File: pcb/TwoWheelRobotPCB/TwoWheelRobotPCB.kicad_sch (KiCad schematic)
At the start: 30 parts, among them J1 Motor1, J2 Motor2, J3 L298n_sense_connector, J4 ACS712_connector, U1 NodeMCU1.0(ESP-12E), U2 L298HN, U3 ACS712_M1, U4 TXB0104D, U5 ACS712_M2, U6 MCP3004

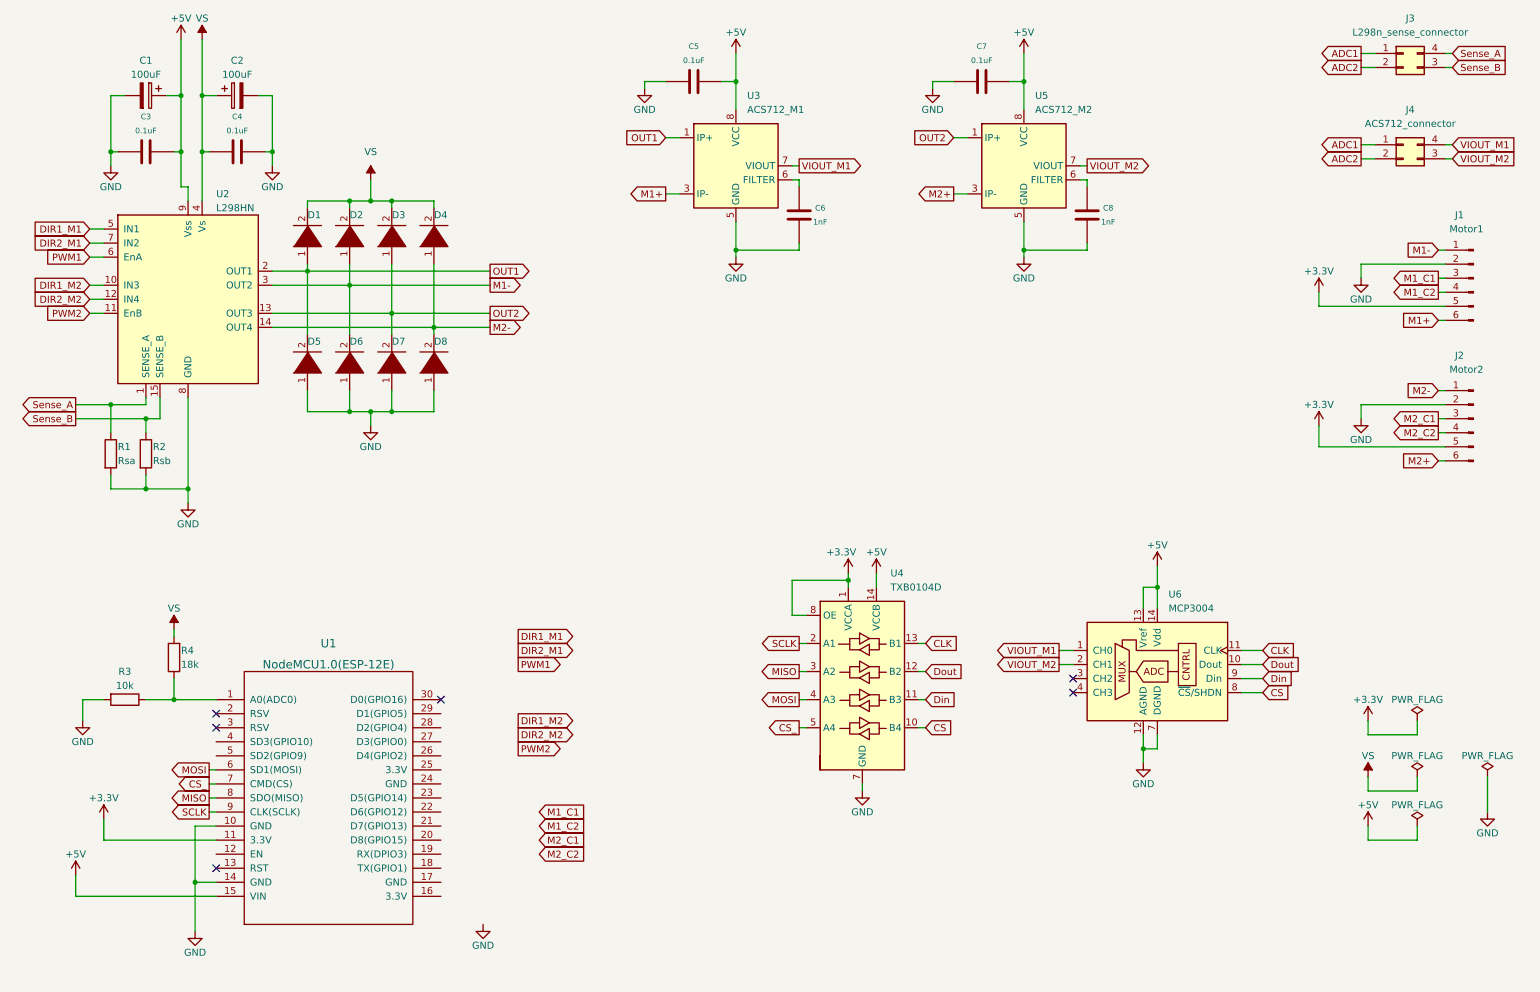
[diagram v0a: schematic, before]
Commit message: pcb update
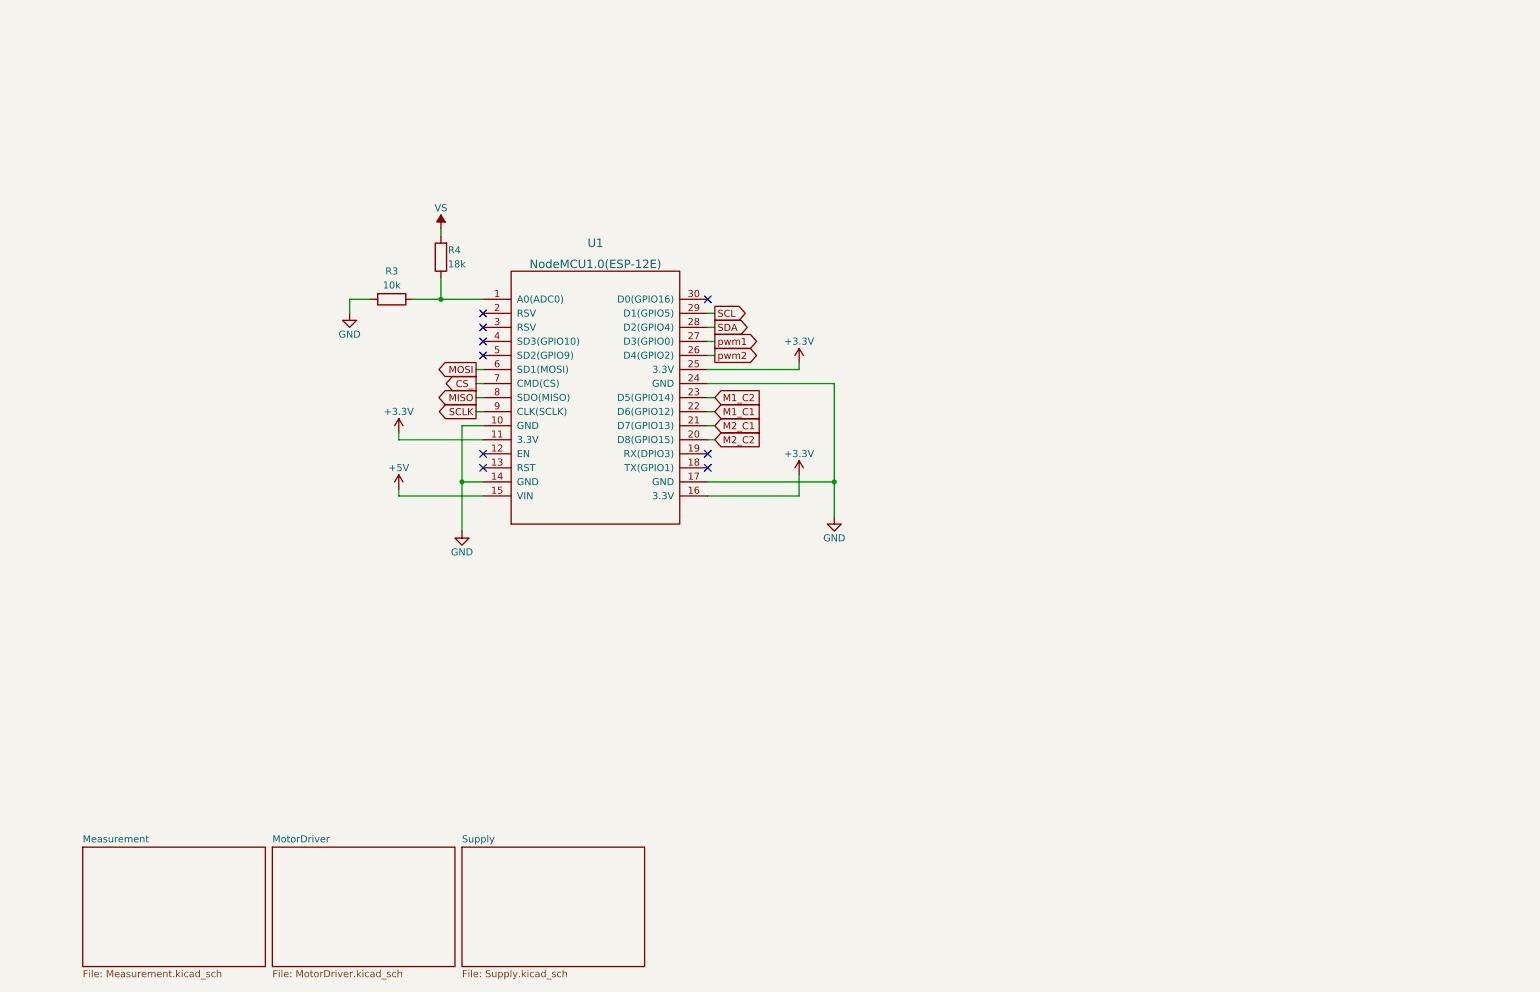
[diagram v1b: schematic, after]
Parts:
- removed C1, C2: 100uF, symbol Device:C_Polarized
- removed C3, C4, C5, C7: 0.1uF, symbol cyclophone:C
- removed C6, C8: 1nF, symbol cyclophone:C
- removed D1, D2, D3, D4, D5, D6, D7, D8: DIODE, symbol pspice:DIODE
- removed J1: Motor1, Connector_PinHeader_2.54mm:PinHeader_1x06_P2.54mm_Vertical, symbol Connector:Conn_01x06_Male
- removed J2: Motor2, Connector_PinHeader_2.54mm:PinHeader_1x06_P2.54mm_Vertical, symbol Connector:Conn_01x06_Male
- removed J3: L298n_sense_connector, Connector_PinHeader_2.54mm:PinHeader_2x02_P2.54mm_Vertical, symbol Connector_Generic:Conn_02x02_Counter_Clockwise
- removed J4: ACS712_connector, Connector_PinHeader_2.54mm:PinHeader_2x02_P2.54mm_Vertical, symbol Connector_Generic:Conn_02x02_Counter_Clockwise
- removed R1: Rsa, symbol Device:R
- removed R2: Rsb, symbol Device:R
- removed U2: L298HN, Package_TO_SOT_THT:TO-220-15_P2.54x2.54mm_StaggerOdd_Lead4.58mm_Vertical, symbol Driver_Motor:L298HN
- removed U3: ACS712_M1, Package_SO:SOIC-8_3.9x4.9mm_P1.27mm, symbol Sensor_Current:ACS712xLCTR-05B
- removed U4: TXB0104D, Package_SO:SOIC-14_3.9x8.7mm_P1.27mm, symbol Logic_LevelTranslator:TXB0104D
- removed U5: ACS712_M2, Package_SO:SOIC-8_3.9x4.9mm_P1.27mm, symbol Sensor_Current:ACS712xLCTR-05B
- removed U6: MCP3004, symbol Analog_ADC:MCP3004
- R3, R4: footprint (none) -> Resistor_SMD:R_0805_2012Metric
- U1: footprint (none) -> NodemcuESP8266_footprint:MODULE_ZC563900
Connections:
- net +3V3: now also U1.16 (3.3V), U1.25 (3.3V)
- net GND: now also U1.17 (GND), U1.24 (GND)
- net M1_C1: now also U1.22 (D6(GPIO12))
- net M1_C2: now also U1.23 (D5(GPIO14))
- net M2_C1: now also U1.21 (D7(GPIO13))
- net M2_C2: now also U1.20 (D8(GPIO15))
- net pwm2: now reaches U1.26 (D4(GPIO2))
- net pwm1: now reaches U1.27 (D3(GPIO0))
- net SDA: now reaches U1.28 (D2(GPIO4))
- net SCL: now reaches U1.29 (D1(GPIO5))
- no-connect marks 6 -> 9
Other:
- added sheet Measurement (Measurement.kicad_sch)
- added sheet MotorDriver (MotorDriver.kicad_sch)
- added sheet Supply (Supply.kicad_sch)
- moved on the sheet: R3, R4, U1

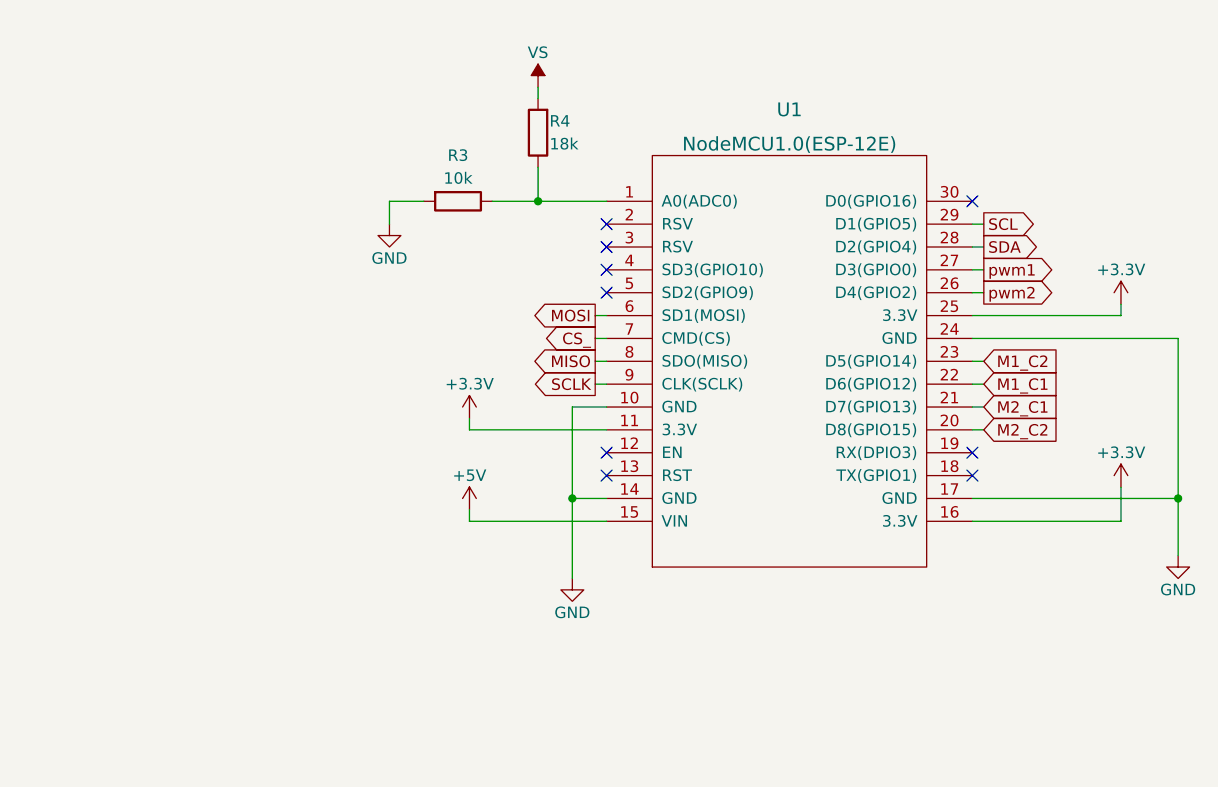
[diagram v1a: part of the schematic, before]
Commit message: update pcb
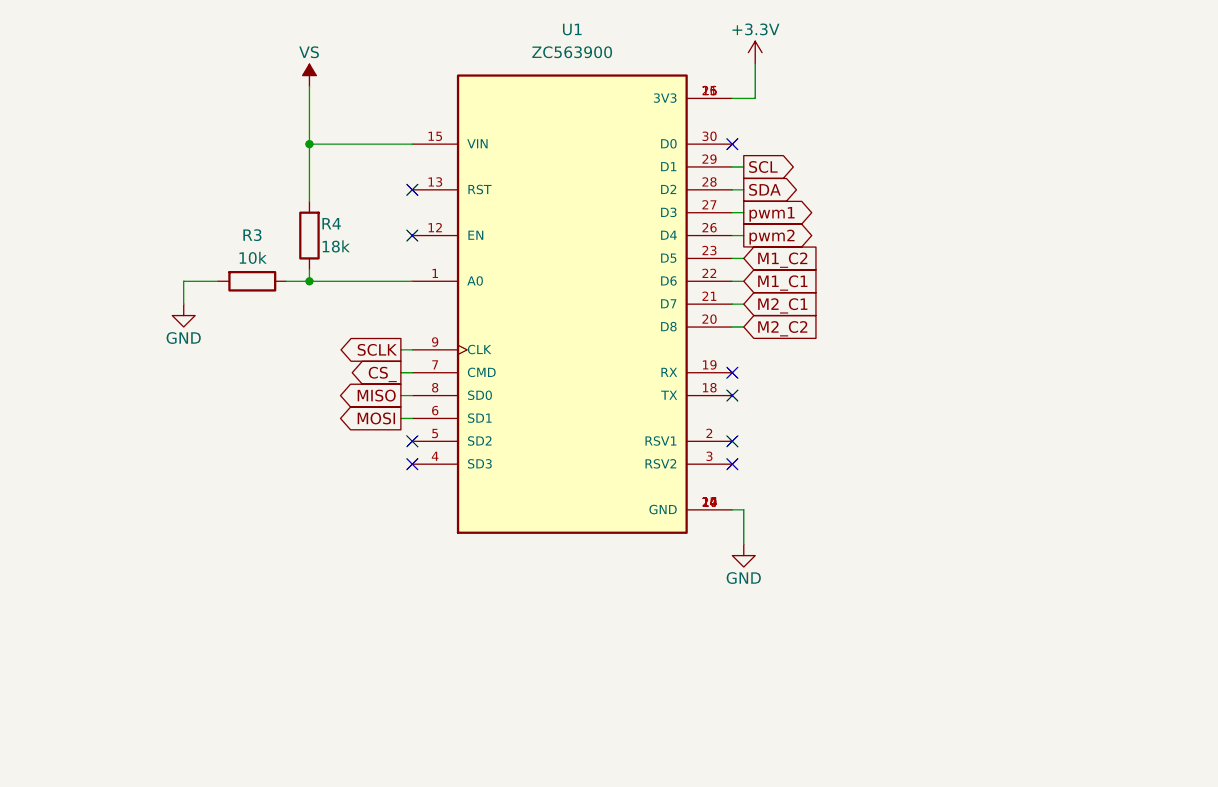
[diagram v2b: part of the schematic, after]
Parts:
- removed U1: NodeMCU1.0(ESP-12E), NodemcuESP8266_footprint:MODULE_ZC563900, symbol ESP8266:NodeMCU1.0(ESP-12E)
- added U1: ZC563900, NodemcuESP8266_footprint:MODULE_ZC563900, symbol NodemcuV2:ZC563900
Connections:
- net +3V3: now also U1.11 (3V3), U1.16 (3V3), U1.25 (3V3)
- net CS_: now also U1.7 (CMD)
- net GND: now also U1.10 (GND), U1.14 (GND), U1.17 (GND), U1.24 (GND)
- net M1_C1: now also U1.22 (D6)
- net M1_C2: now also U1.23 (D5)
- net M2_C1: now also U1.21 (D7)
- net M2_C2: now also U1.20 (D8)
- net MISO: now also U1.8 (SD0)
- net MOSI: now also U1.6 (SD1)
- net SCL: now also U1.29 (D1)
- net SCLK: now also U1.9 (CLK)
- net SDA: now also U1.28 (D2)
- net VS: now also U1.15 (VIN)
- net pwm1: now also U1.27 (D3)
- net pwm2: now also U1.26 (D4)
- net at R3.1, R4.1: now also U1.1 (A0)
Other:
- moved on the sheet: R3, R4

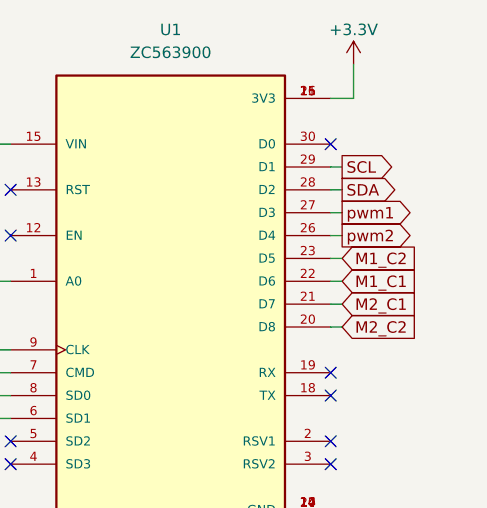
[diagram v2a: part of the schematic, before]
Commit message: pcb
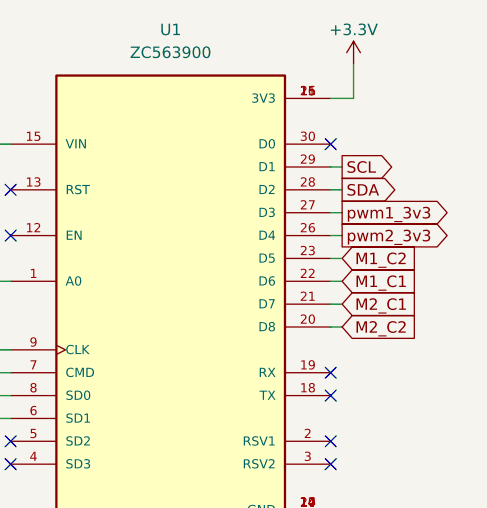
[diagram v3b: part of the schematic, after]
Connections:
- net pwm1 renamed pwm1_3v3
- net pwm2 renamed pwm2_3v3
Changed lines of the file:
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@@
     )
   )
-  (global_label "pwm2" (shape output) (at 111.76 69.85 0) (fields_autoplaced)
+  (global_label "pwm2_3v3" (shape output) (at 111.76 69.85 0) (fields_autoplaced)
     (effects (font (size 1.27 1.27)) (justify left))
-    (property "Intersheet References" "${INTERSHEET_REFS}" (id 0) (at 119.5555 69.7706 0)
+    (property "Intersheet References" "${INTERSHEET_REFS}" (id 0) (at 123.9098 69.7706 0)
       (effects (font (size 1.27 1.27)) (justify left) hide)
     )
@@
     )
   )
-  (global_label "pwm1" (shape output) (at 111.76 67.31 0) (fields_autoplaced)
+  (global_label "pwm1_3v3" (shape output) (at 111.76 67.31 0) (fields_autoplaced)
     (effects (font (size 1.27 1.27)) (justify left))
-    (property "Intersheet References" "${INTERSHEET_REFS}" (id 0) (at 119.5555 67.2306 0)
+    (property "Intersheet References" "${INTERSHEET_REFS}" (id 0) (at 123.9098 67.2306 0)
       (effects (font (size 1.27 1.27)) (justify left) hide)
     )
@@
       (reference "#FLG04") (unit 1) (value "PWR_FLAG") (footprint "")
     )
+    (path "/7d587865-2231-4a38-9d8a-97d485f2f4e4/4c8df18d-77ed-4411-bc03-a1485170a702"
+      (reference "#PWR01") (unit 1) (value "VS") (footprint "")
+    )
     (path "/a80922d8-842d-4acc-a603-f8902aa0c0c5"
       (reference "#PWR02") (unit 1) (value "GND") (footprint "")
     )
+    (path "/7d587865-2231-4a38-9d8a-97d485f2f4e4/984e7252-4d51-4e18-8cfd-d20f5368238e"
+      (reference "#PWR03") (unit 1) (value "GND") (footprint "")
+    )
+    (path "/7d587865-2231-4a38-9d8a-97d485f2f4e4/cbc1633b-2edb-4841-a64c-00ea63fa9a87"
+      (reference "#PWR04") (unit 1) (value "VS") (footprint "")
+    )
     (path "/bab16bbd-be5b-4ff6-9805-0a16f023b621"
       (reference "#PWR05") (unit 1) (value "VS") (footprint "")
     )
+    (path "/7d587865-2231-4a38-9d8a-97d485f2f4e4/df76744a-2672-4df3-b0f1-8632a1e0c956"
+      (reference "#PWR06") (unit 1) (value "GND") (footprint "")
+    )
+    (path "/7d587865-2231-4a38-9d8a-97d485f2f4e4/15eb6ae6-6d8f-499f-a0b3-7ad0e61d54f9"
+      (reference "#PWR07") (unit 1) (value "GND") (footprint "")
+    )
     (path "/5d98914d-1801-43c8-96ca-19f222dbae40/43f9481c-710c-4a70-b5b4-8f4b24641629"
       (reference "#PWR08") (unit 1) (value "GND") (footprint "")
@@
       (reference "#PWR011") (unit 1) (value "VS") (footprint "")
     )
+    (path "/7d587865-2231-4a38-9d8a-97d485f2f4e4/d045e7ba-b7a5-4eb8-ba31-1a87a3b8ae7d"
+      (reference "#PWR012") (unit 1) (value "+5V") (footprint "")
+    )
     (path "/5d98914d-1801-43c8-96ca-19f222dbae40/30c9f8d1-6270-4c18-a2b6-c43a30582ae1"
       (reference "#PWR013") (unit 1) (value "GND") (footprint "")
@@
       (reference "#PWR019") (unit 1) (value "GND") (footprint "")
     )
-    (path "/5d98914d-1801-43c8-96ca-19f222dbae40/47165815-d55a-454b-961f-9380e65de16a"
+    (path "/5d98914d-1801-43c8-96ca-19f222dbae40/e3cbd370-7c22-4222-878e-9ad9b35baaf2"
       (reference "#PWR020") (unit 1) (value "+3.3V") (footprint "")
     )
-    (path "/5d98914d-1801-43c8-96ca-19f222dbae40/e457ae7e-3438-4d1d-a954-7f6d6264bc05"
-      (reference "#PWR021") (unit 1) (value "GND") (footprint "")
-    )
-    (path "/5d98914d-1801-43c8-96ca-19f222dbae40/d657a5c7-f508-4351-b8c0-caf046b97c66"
-      (reference "#PWR022") (unit 1) (value "+5V") (footprint "")
+    (path "/5d98914d-1801-43c8-96ca-19f222dbae40/11b85eea-dc35-46a9-96f1-4b1e7636e86a"
+      (reference "#PWR021") (unit 1) (value "+3.3V") (footprint "")
+    )
+    (path "/5d98914d-1801-43c8-96ca-19f222dbae40/2bf65490-bdce-49a7-b615-e71bdc3e6432"
+      (reference "#PWR022") (unit 1) (value "GND") (footprint "")
     )
     (path "/5d98914d-1801-43c8-96ca-19f222dbae40/446365ea-1547-4ab1-9f38-dd7104295afb"
@@
       (reference "#PWR041") (unit 1) (value "GND") (footprint "")
     )
+    (path "/5d98914d-1801-43c8-96ca-19f222dbae40/fd4dabcb-18d2-466b-b827-05bda2ed2a9c"
+      (reference "#PWR042") (unit 1) (value "+5V") (footprint "")
+    )
     (path "/1862457e-eb7f-42c4-b8ca-a4b27406c6d7"
       (reference "#PWR0101") (unit 1) (value "GND") (footprint "")
@@
       (reference "C8") (unit 1) (value "1nF") (footprint "Capacitor_SMD:C_0805_2012Metric")
     )
+    (path "/7d587865-2231-4a38-9d8a-97d485f2f4e4/8c56c79c-7af4-40fc-8d6c-2391d30538c4"
+      (reference "C9") (unit 1) (value "100uF") (footprint "Capacitor_THT:CP_Radial_D6.3mm_P2.50mm")
+    )
+    (path "/7d587865-2231-4a38-9d8a-97d485f2f4e4/90f4a887-faea-4c69-a0af-0d8fe86d677c"
+      (reference "C10") (unit 1) (value "0.1uF") (footprint "Capacitor_THT:C_Disc_D4.3mm_W1.9mm_P5.00mm")
+    )
+    (path "/7d587865-2231-4a38-9d8a-97d485f2f4e4/21a0e9c8-dee6-4f28-bdc4-f2405df583e6"
+      (reference "C11") (unit 1) (value "680uF") (footprint "Capacitor_SMD:CP_Elec_8x6.9")
+    )
+    (path "/7d587865-2231-4a38-9d8a-97d485f2f4e4/0ae213ea-5f39-486e-886a-e2700d74a572"
+      (reference "C12") (unit 1) (value "220uF") (footprint "Capacitor_SMD:CP_Elec_8x6.9")
+    )
     (path "/5d98914d-1801-43c8-96ca-19f222dbae40/ea2db8f6-2cca-4218-9b19-60965fcb02ed"
       (reference "D1") (unit 1) (value "DIODE") (footprint "Diode_THT:D_A-405_P10.16mm_Horizontal")
@@
       (reference "D8") (unit 1) (value "DIODE") (footprint "Diode_THT:D_A-405_P10.16mm_Horizontal")
     )
+    (path "/7d587865-2231-4a38-9d8a-97d485f2f4e4/52ef34a6-f506-464a-95e4-48addca555bc"
+      (reference "D9") (unit 1) (value "1N5825") (footprint "Diode_SMD:D_2010_5025Metric_Pad1.52x2.65mm_HandSolder")
+    )
     (path "/5d98914d-1801-43c8-96ca-19f222dbae40/ad439bee-fa7a-4275-9dda-be9562a285ae"
-      (reference "J3") (unit 1) (value "Motor1") (footprint "Connector_PinHeader_2.54mm:PinHeader_1x06_P2.54mm_Vertical")
+      (reference "J1") (unit 1) (value "Motor1") (footprint "Connector_PinHeader_2.54mm:PinHeader_1x06_P2.54mm_Vertical")
     )
     (path "/5d98914d-1801-43c8-96ca-19f222dbae40/42d8d183-8a6d-45ba-a12d-bbab6eb9317f"
-      (reference "J4") (unit 1) (value "Motor2") (footprint "Connector_PinHeader_2.54mm:PinHeader_1x06_P2.54mm_Vertical")
+      (reference "J2") (unit 1) (value "Motor2") (footprint "Connector_PinHeader_2.54mm:PinHeader_1x06_P2.54mm_Vertical")
+    )
+    (path "/7d587865-2231-4a38-9d8a-97d485f2f4e4/b0999983-8823-4164-8436-8bf2e6297058"
+      (reference "J3") (unit 1) (value "POWER") (footprint "TerminalBlock_RND:TerminalBlock_RND_205-00001_1x02_P5.00mm_Horizontal")
+    )
+    (path "/7d587865-2231-4a38-9d8a-97d485f2f4e4/5379c07b-65c8-4496-8da0-933e8b8a86a5"
+      (reference "J4") (unit 1) (value "XT60-M") (footprint "footprint:AMASS_XT60-M")
+    )
+    (path "/7d587865-2231-4a38-9d8a-97d485f2f4e4/c665d5f5-cfa3-4d27-ba71-29f466dc52e9"
+      (reference "L1") (unit 1) (value "33uH") (footprint "Inductor_SMD:L_Bourns_SRP1245A")
     )
     (path "/5d98914d-1801-43c8-96ca-19f222dbae40/e6024f9f-8e68-45e7-a471-d53cf11ecf66"
@@
       (reference "R6") (unit 1) (value "2k2") (footprint "Resistor_SMD:R_0805_2012Metric")
     )
+    (path "/7d587865-2231-4a38-9d8a-97d485f2f4e4/1495b4af-d2d5-4440-8b78-75857f825242"
+      (reference "SW1") (unit 1) (value "SW_DPDT_x2") (footprint "Button_Switch_THT:SW_PUSH_E-Switch_FS5700DP_DPDT")
+    )
     (path "/ec062509-e43d-478c-ad0a-4deb2e0e42c0"
       (reference "U1") (unit 1) (value "ZC563900") (footprint "NodemcuESP8266_footprint:MODULE_ZC563900")
@@
       (reference "U3") (unit 1) (value "PCF8574") (footprint "PCF8574:SO16W")
     )
-    (path "/5d98914d-1801-43c8-96ca-19f222dbae40/8af2360a-9a89-4a36-a9b6-da5a660b1e19"
-      (reference "U4") (unit 1) (value "TXB0108DQSR") (footprint "TXB0108_TSOP20_fotprint:SOP65P640X120-20N")
+    (path "/5d98914d-1801-43c8-96ca-19f222dbae40/cd676e39-8b0b-4a97-a5f7-f1a894ba4f9c"
+      (reference "U4") (unit 1) (value "TXB0108PWR") (footprint "TXB0108_TSOP20_fotprint:SOP65P640X120-20N")
     )
     (path "/4f34e6bd-8488-4666-87ea-d049bdfdbeee/1c670057-d2d9-4caa-afa0-cbbef1da2910"
@@
       (reference "U8") (unit 1) (value "ACS712_M2") (footprint "Package_SO:SOIC-8_3.9x4.9mm_P1.27mm")
     )
-  )
+    (path "/7d587865-2231-4a38-9d8a-97d485f2f4e4/faecffa1-e510-4609-90b1-ec816da7b5c8"
+      (reference "U9") (unit 1) (value "LM2596S-5") (footprint "Package_TO_SOT_SMD:TO-263-5_TabPin3")
+    )
+  )
